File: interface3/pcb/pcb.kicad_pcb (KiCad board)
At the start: 4 copper layers, 65 x 55 mm, 27 parts, among them J1 Conn_Coaxial, T1 Murata 78602/8JC, U1 DS34LV86T, U2 DS34LV87T, U3 Pico_W

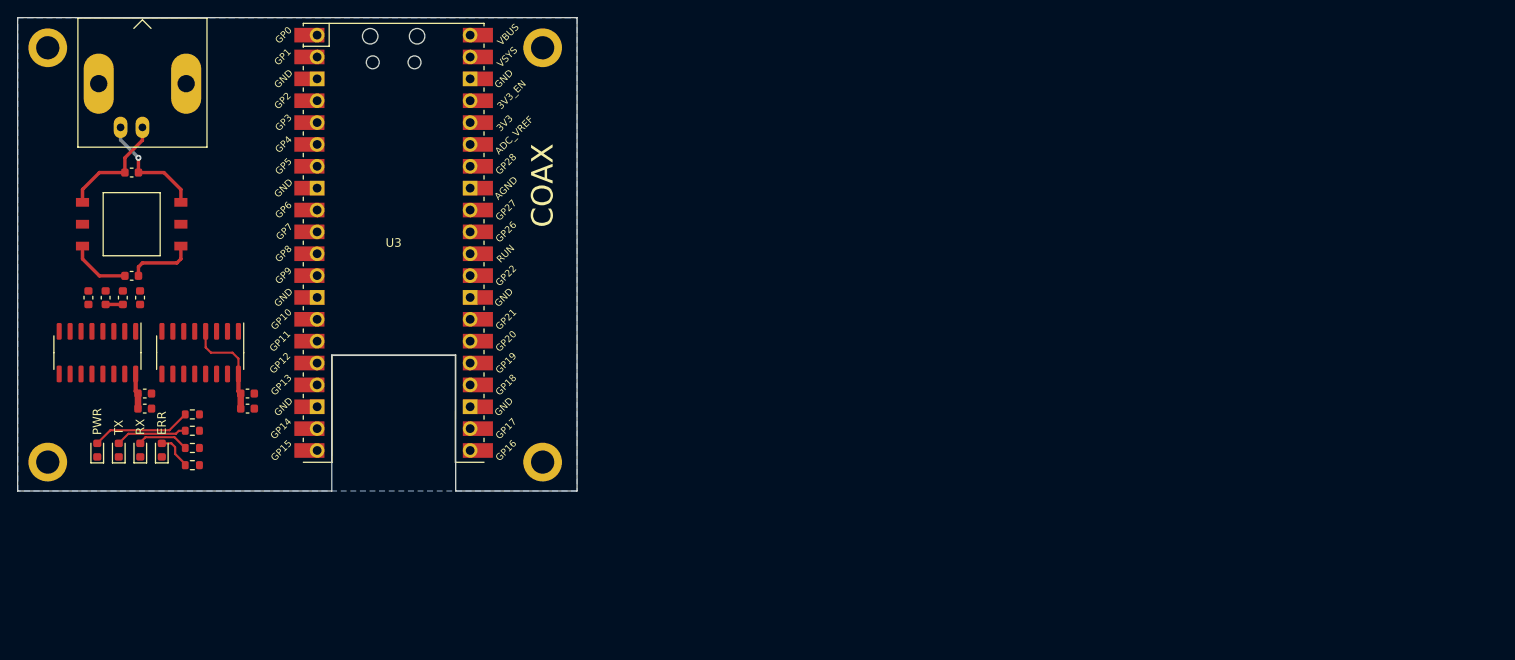
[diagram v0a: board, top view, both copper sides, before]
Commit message: pcb work
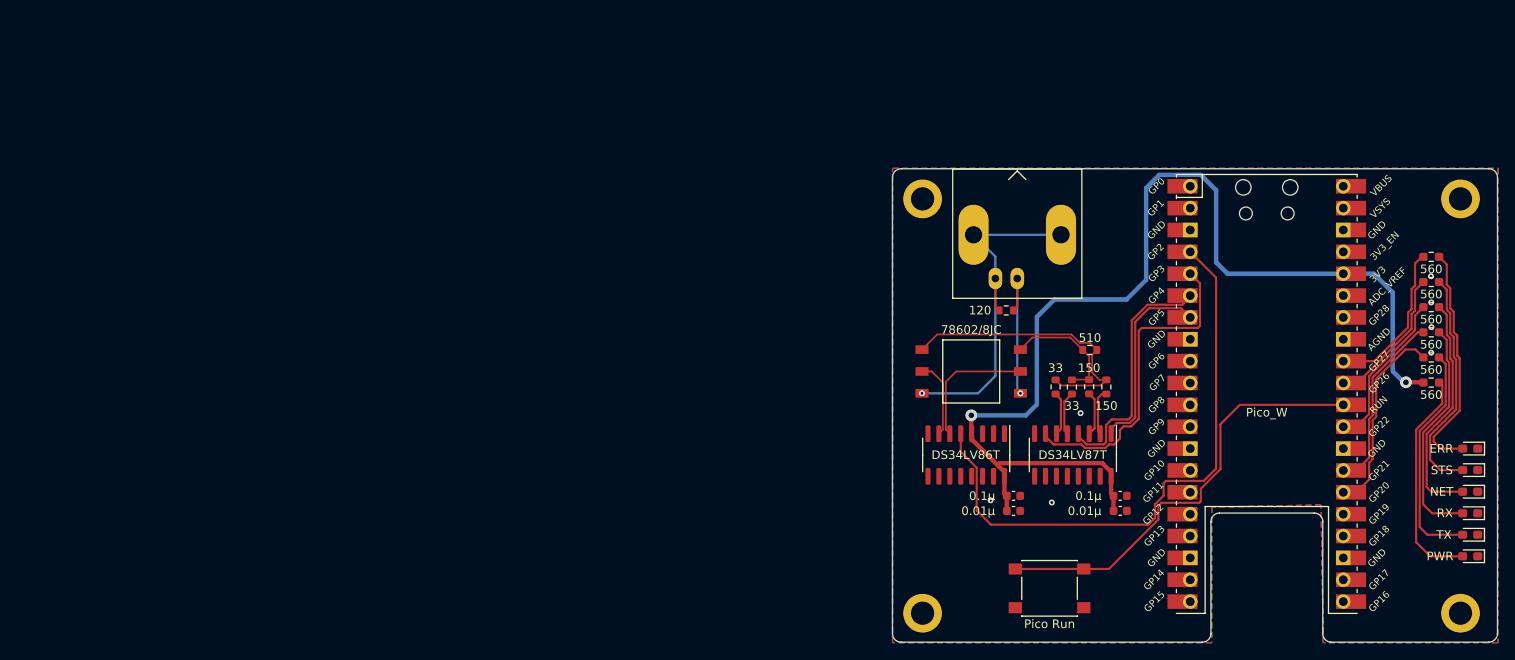
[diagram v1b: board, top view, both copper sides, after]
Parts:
- removed R16: 560, Resistor_SMD:R_0603_1608Metric
- added D5: STS, LED_SMD:LED_0603_1608Metric_Pad1.05x0.95mm_HandSolder, F.Cu at (185.5, 112.8)
- added D6: ERR, LED_SMD:LED_0603_1608Metric_Pad1.05x0.95mm_HandSolder, F.Cu at (185.5, 110.3)
- added R10: 560, Resistor_SMD:R_0603_1608Metric_Pad0.98x0.95mm_HandSolder, F.Cu at (181.0, 99.7)
- added R7: 560, Resistor_SMD:R_0603_1608Metric_Pad0.98x0.95mm_HandSolder, F.Cu at (181.0, 91.0)
- added R9: 560, Resistor_SMD:R_0603_1608Metric_Pad0.98x0.95mm_HandSolder, F.Cu at (181.0, 88.0)
- added SW1: Pico Run, Button_Switch_SMD:SW_Push_1P1T_NO_6x6mm_H9.5mm, F.Cu at (136.6, 126.6)
- C1, C2: value 0.1uF -> 0.1µ
- C3, C4: value 0.01uF -> 0.01µ
- D1: value GRN -> PWR; footprint LED_SMD:LED_0603_1608Metric -> LED_SMD:LED_0603_1608Metric_Pad1.05x0.95mm_HandSolder
- D2: value YEL -> TX; footprint LED_SMD:LED_0603_1608Metric -> LED_SMD:LED_0603_1608Metric_Pad1.05x0.95mm_HandSolder
- D3: value YEL -> RX; footprint LED_SMD:LED_0603_1608Metric -> LED_SMD:LED_0603_1608Metric_Pad1.05x0.95mm_HandSolder
- D4: value RED -> NET; footprint LED_SMD:LED_0603_1608Metric -> LED_SMD:LED_0603_1608Metric_Pad1.05x0.95mm_HandSolder
- R11, R12, R8: footprint Resistor_SMD:R_0603_1608Metric -> Resistor_SMD:R_0603_1608Metric_Pad0.98x0.95mm_HandSolder
- T1: value Murata 78602/8JC -> 78602/8JC
- moved D1 160.0 mm to (185.5, 122.8), turned to 180 degrees
- moved D2 157.3 mm to (185.5, 120.3), turned to 180 degrees
- moved D3 154.7 mm to (185.5, 117.8), turned to 180 degrees
- moved D4 152.1 mm to (185.5, 115.3), turned to 180 degrees
- moved R12 144.9 mm to (181.0, 93.9), turned to 0 degrees
- moved R11 144.4 mm to (181.0, 96.8), turned to 0 degrees
- moved R8 144.0 mm to (181.0, 102.7), turned to 0 degrees
- moved R2 118.7 mm to (143.2, 103.2), turned to 90 degrees
- moved R1 114.7 mm to (141.2, 103.1), turned to -90 degrees
- moved C2 114.0 mm to (144.9, 115.8)
- moved C4 114.0 mm to (144.9, 117.6)
- moved U2 114.0 mm to (139.4, 111.1)
- moved R5 111.7 mm to (141.3, 98.9)
- moved R3 110.8 mm to (139.2, 103.2), turned to -90 degrees
- moved H1 108.1 mm to (184.4, 81.3)
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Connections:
- R11 pad 1: ~{TX} -> LED_RX
- R11 pad 2: Net-(D2-A) -> Net-(D3-A)
- R12 pad 1: RX -> LED_NET
- R12 pad 2: Net-(D3-A) -> Net-(D4-A)
- R8 pad 1: LED_STATUS -> +3V3
- U3 pad 10: LED_ERROR -> unconnected-(U3-GPIO7-Pad10)
- U3 pad 11: LED_STATUS -> unconnected-(U3-GPIO8-Pad11)
- U3 pad 26: unconnected-(U3-GPIO20-Pad26) -> LED_TX
- U3 pad 27: unconnected-(U3-GPIO21-Pad27) -> LED_RX
- U3 pad 29: unconnected-(U3-GPIO22-Pad29) -> LED_NET
- U3 pad 30: unconnected-(U3-RUN-Pad30) -> PICO_RUN
- U3 pad 31: unconnected-(U3-GPIO26_ADC0-Pad31) -> LED_STS
- U3 pad 32: unconnected-(U3-GPIO27_ADC1-Pad32) -> LED_ERR
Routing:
- net +3V3: track 16.3 -> 127.7 mm, vias 0 -> 2
- net RX: track 0.00 -> 69.1 mm
- net PICO_RUN: track 0.00 -> 50.8 mm
- net ~{TX}: track 0.00 -> 37.8 mm
- net TX_ACTIVE: track 0.00 -> 28.6 mm
- net Net-(J1-Ext): track 13.3 -> 40.9 mm
- net Net-(D6-A): track 0.00 -> 27.4 mm
- net Net-(D5-A): track 0.00 -> 27.0 mm
- net TX-: track 7.84 -> 33.1 mm
- net LED_TX: track 0.00 -> 22.9 mm
- net Net-(D4-A): track 4.49 -> 27.2 mm
- net TX_DELAY: track 0.00 -> 22.5 mm
- net LED_RX: track 0.00 -> 21.2 mm
- net Net-(D3-A): track 6.11 -> 26.7 mm
- net LED_NET: track 0.00 -> 18.6 mm
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- added copper zone on F.Cu, net GND
- removed copper zone on In2.Cu, net +3V3
- removed copper zone on In1.Cu, net GND
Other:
- board size 65 x 55 mm -> 70.3 x 55 mm
- copper layers 4 -> 2
- board text removed: "COAX"
- board text removed: "ERR"
- board text removed: "PWR"
- board text removed: "RX"
- board text removed: "TX"
